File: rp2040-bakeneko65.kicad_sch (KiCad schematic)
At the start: 11 parts, among them SW1 SW_Push, U1 W25Q128JVS, U3 RP2040, Y1 12MHz

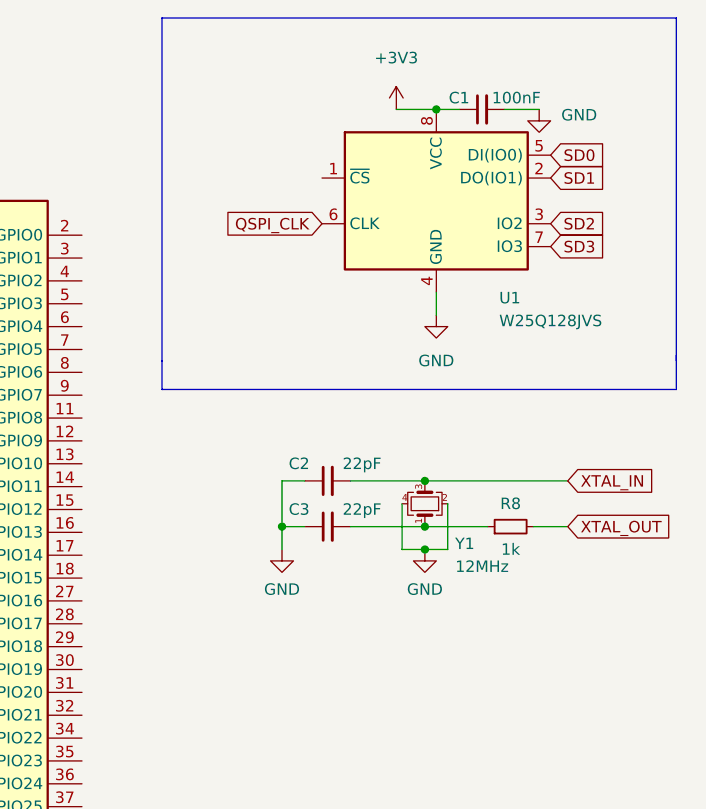
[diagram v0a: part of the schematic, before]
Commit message: Some line stuff
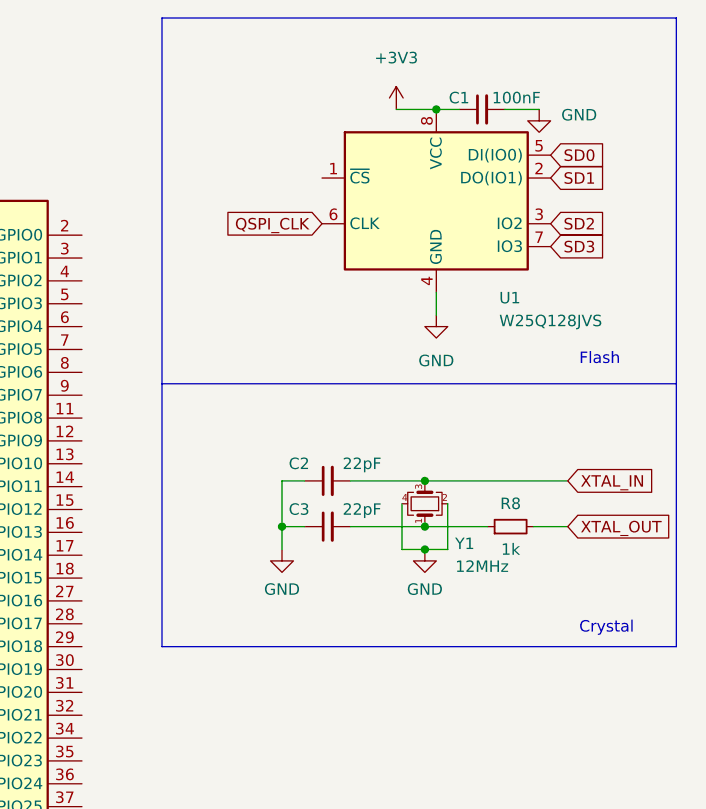
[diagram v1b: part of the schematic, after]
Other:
- note added: "Crystal"
- note added: "Flash"
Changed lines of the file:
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@@
     (stroke (width 0) (type default) (color 0 0 0 0))
+  )
+  (polyline (pts (xy 165.1 53.34) (xy 107.95 53.34))
+    (stroke (width 0) (type solid) (color 0 0 0 0))
   )
   (wire (pts (xy 76.2 26.67) (xy 76.2 29.21))
@@
     (stroke (width 0) (type default) (color 0 0 0 0))
   )
-  (polyline (pts (xy 107.95 12.7) (xy 165.1 12.7))
-    (stroke (width 0) (type solid) (color 0 0 0 0))
-  )
-  (polyline (pts (xy 165.1 53.975) (xy 107.95 53.975))
-    (stroke (width 0) (type solid) (color 0 0 0 0))
-  )
   (wire (pts (xy 139.7 71.755) (xy 137.16 71.755))
     (stroke (width 0) (type default) (color 0 0 0 0))
@@
     (stroke (width 0) (type default) (color 0 0 0 0))
   )
+  (polyline (pts (xy 107.95 53.34) (xy 107.95 82.55))
+    (stroke (width 0) (type solid) (color 0 0 0 0))
+  )
   (wire (pts (xy 46.99 31.75) (xy 46.99 36.83))
     (stroke (width 0) (type default) (color 0 0 0 0))
-  )
-  (polyline (pts (xy 165.1 12.7) (xy 165.1 50.8))
-    (stroke (width 0) (type solid) (color 0 0 0 0))
   )
   (wire (pts (xy 123.825 69.215) (xy 121.285 69.215))
@@
     (stroke (width 0) (type default) (color 0 0 0 0))
   )
+  (polyline (pts (xy 165.1 53.34) (xy 165.1 82.55))
+    (stroke (width 0) (type solid) (color 0 0 0 0))
+  )
   (wire (pts (xy 138.43 22.86) (xy 140.97 22.86))
     (stroke (width 0) (type default) (color 0 0 0 0))
@@
   (wire (pts (xy 128.905 64.135) (xy 137.16 64.135))
     (stroke (width 0) (type default) (color 0 0 0 0))
+  )
+  (polyline (pts (xy 107.95 12.7) (xy 165.1 12.7))
+    (stroke (width 0) (type solid) (color 0 0 0 0))
   )
   (wire (pts (xy 138.43 43.18) (xy 138.43 45.72))
@@
     (stroke (width 0) (type default) (color 0 0 0 0))
   )
-  (polyline (pts (xy 165.1 50.165) (xy 165.1 53.975))
-    (stroke (width 0) (type solid) (color 0 0 0 0))
-  )
   (wire (pts (xy 121.285 64.135) (xy 123.825 64.135))
     (stroke (width 0) (type default) (color 0 0 0 0))
@@
     (stroke (width 0) (type default) (color 0 0 0 0))
   )
+  (polyline (pts (xy 107.95 53.34) (xy 107.95 12.7))
+    (stroke (width 0) (type solid) (color 0 0 0 0))
+  )
   (wire (pts (xy 43.18 113.03) (xy 48.26 113.03))
     (stroke (width 0) (type default) (color 0 0 0 0))
@@
   (wire (pts (xy 81.28 29.21) (xy 83.82 29.21))
     (stroke (width 0) (type default) (color 0 0 0 0))
-  )
-  (polyline (pts (xy 107.95 12.7) (xy 107.95 50.8))
-    (stroke (width 0) (type solid) (color 0 0 0 0))
   )
   (wire (pts (xy 43.18 46.99) (xy 48.26 46.99))
@@
     (stroke (width 0) (type default) (color 0 0 0 0))
   )
-  (polyline (pts (xy 107.95 53.975) (xy 107.95 50.8))
-    (stroke (width 0) (type solid) (color 0 0 0 0))
-  )
   (wire (pts (xy 68.58 26.67) (xy 68.58 29.21))
     (stroke (width 0) (type default) (color 0 0 0 0))
+  )
+  (polyline (pts (xy 165.1 12.7) (xy 165.1 53.34))
+    (stroke (width 0) (type solid) (color 0 0 0 0))
   )
   (wire (pts (xy 44.45 36.83) (xy 46.99 36.83))
@@
     (stroke (width 0) (type default) (color 0 0 0 0))
   )
+  (polyline (pts (xy 165.1 82.55) (xy 107.95 82.55))
+    (stroke (width 0) (type solid) (color 0 0 0 0))
+  )
+  (text "Flash\n" (at 154.305 51.435 0)
+    (effects (font (size 1.27 1.27)) (justify left bottom))
+  )
+  (text "Crystal" (at 154.305 81.28 0)
+    (effects (font (size 1.27 1.27)) (justify left bottom))
+  )
   (global_label "XTAL_OUT" (shape input) (at 45.72 92.71 180) (fields_autoplaced)
